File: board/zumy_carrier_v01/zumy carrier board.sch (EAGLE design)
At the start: 22 parts, among them IC1 SN74AUP2G17, IC2 SN74AUP2G17, J1 ODROID_POWER, J2 BATT_POWER, M2 ITG/MPU_MODULE, M3 POLOLU_DRV8833_MODULE, SW1 500SSP1S1M6QEA

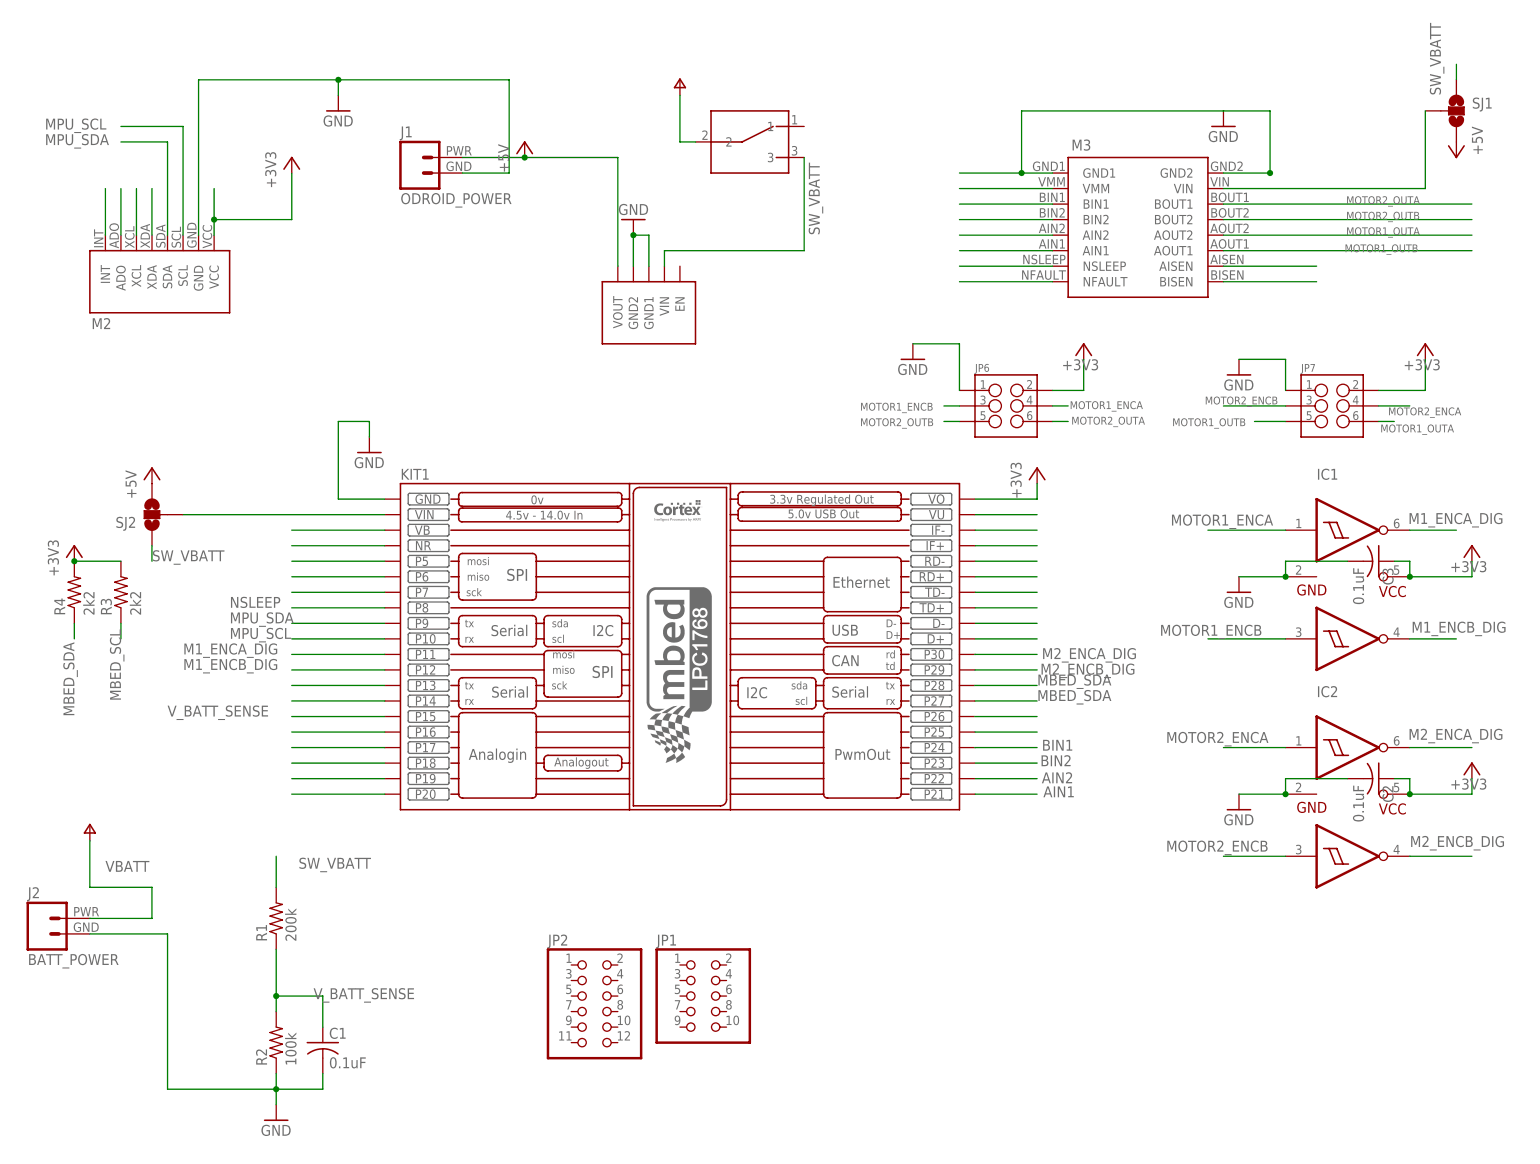
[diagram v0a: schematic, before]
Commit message: First pass at layout done
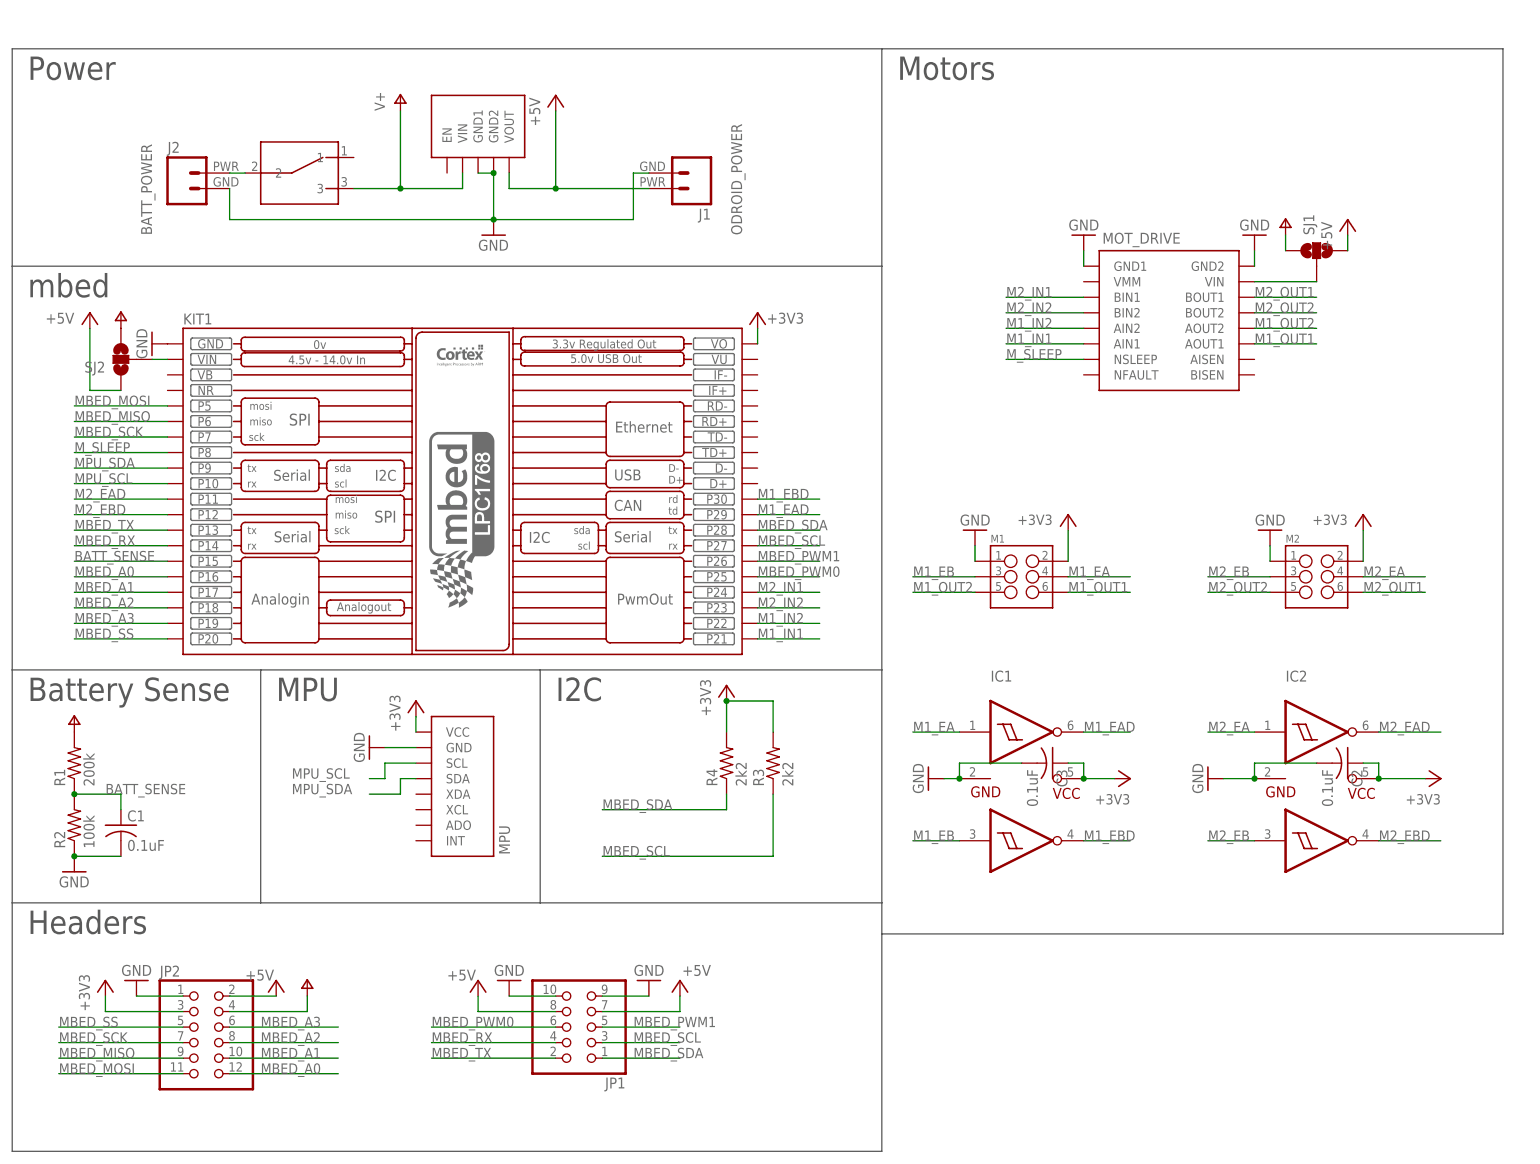
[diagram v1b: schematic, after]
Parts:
- removed JP6, JP7: (no value), SparkFun-Connectors:M03X2SHROUD
- removed M3: POLOLU_DRV8833_MODULE, zumy:POLOLU_DRV8833_MODULE
- added M1: (no value), SparkFun-Connectors:M03X2SHROUD
- added MOT_DRIVE: POLOLU_DRV8833_MODULE, zumy:POLOLU_DRV8833_MODULE
- added MPU: ITG/MPU_MODULE, zumy:ITG/MPU_MODULE
- M2: value ITG/MPU_MODULE -> (none); device zumy:ITG/MPU_MODULE -> SparkFun-Connectors:M03X2SHROUD
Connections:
- net VBATT renamed N$2
- net V_BATT_SENSE renamed BATT_SENSE
- removed net AIN1: KIT1.P21, M3.AIN1
- removed net AIN2: KIT1.P22, M3.AIN2
- removed net BIN1: KIT1.P24, M3.BIN1
- removed net BIN2: KIT1.P23, M3.BIN2
- removed net M1_ENCA_DIG: IC1.1Y, KIT1.P11
- removed net M1_ENCB_DIG: IC1.2Y, KIT1.P12
- removed net M2_ENCA_DIG: IC2.1Y, KIT1.P30
- removed net M2_ENCB_DIG: IC2.2Y, KIT1.P29
- removed net MOTOR1_ENCA: IC1.1A, JP6.4
- removed net MOTOR1_ENCB: IC1.2A, JP6.3
- removed net MOTOR1_OUTA: JP7.6, M3.AOUT2
- removed net MOTOR1_OUTB: JP7.5, M3.AOUT1
- removed net MOTOR2_ENCA: IC2.1A, JP7.4
- removed net MOTOR2_ENCB: IC2.2A, JP7.3
- removed net MOTOR2_OUTA: JP6.6, M3.BOUT1
- removed net MOTOR2_OUTB: JP6.5, M3.BOUT2
- removed net N$1 (its old number): M2.INT
- removed net N$10: KIT1.P16
- removed net N$11: KIT1.VB
- removed net N$12: KIT1.NR
- removed net N$13: KIT1.P5
- removed net N$14: KIT1.P6
- removed net N$15: KIT1.P7
- removed net N$16: M3.VIN, SJ1.2
- removed net N$2 (its old number): M2.ADO
- removed net N$21: KIT1.P13
- removed net N$22: KIT1.P14
- removed net N$25: KIT1.P17
- removed net N$26: KIT1.P18
- removed net N$27: KIT1.P19
- removed net N$33: KIT1.P25
- removed net N$34: KIT1.P26
- removed net N$4: M2.XDA
- removed net N$41: KIT1.TD+
- removed net N$42: KIT1.TD-
- removed net N$43: KIT1.RD+
- removed net N$44: KIT1.RD-
- removed net N$45: KIT1.IF+
- removed net N$46: KIT1.IF-
- removed net N$47: KIT1.VU
- removed net N$5: KIT1.D-
- removed net N$50: M3.VMM
- removed net N$56: M3.NFAULT
- removed net N$6: KIT1.D+
- removed net N$63: M3.AISEN
- removed net N$64: M3.BISEN
- removed net N$7: KIT1.P20
- removed net NSLEEP: KIT1.P8, M3.NSLEEP
- removed net SW_VBATT: R1.2, SJ1.1, SJ2.1, SW1.3, U$5.VIN
- new net M1_EA: IC1.1A, M1.4
- new net M1_EAD: IC1.1Y, KIT1.P29
- new net M1_EB: IC1.2A, M1.3
- new net M1_EBD: IC1.2Y, KIT1.P30
- new net M1_IN1: KIT1.P21, MOT_DRIVE.AIN1
- new net M1_IN2: KIT1.P22, MOT_DRIVE.AIN2
- new net M1_OUT1: M1.6, MOT_DRIVE.AOUT1
- new net M1_OUT2: M1.5, MOT_DRIVE.AOUT2
- new net M2_EA: IC2.1A, M2.4
- new net M2_EAD: IC2.1Y, KIT1.P11
- new net M2_EB: IC2.2A, M2.3
- new net M2_EBD: IC2.2Y, KIT1.P12
- new net M2_IN1: KIT1.P24, MOT_DRIVE.BIN1
- new net M2_IN2: KIT1.P23, MOT_DRIVE.BIN2
- new net M2_OUT1: M2.6, MOT_DRIVE.BOUT1
- new net M2_OUT2: M2.5, MOT_DRIVE.BOUT2
- new net MBED_A0: JP2.12, KIT1.P16
- new net MBED_A1: JP2.10, KIT1.P17
- new net MBED_A2: JP2.8, KIT1.P18
- new net MBED_A3: JP2.6, KIT1.P19
- new net MBED_MISO: JP2.9, KIT1.P6
- new net MBED_MOSI: JP2.11, KIT1.P5
- new net MBED_PWM0: JP1.6, KIT1.P25
- new net MBED_PWM1: JP1.5, KIT1.P26
- new net MBED_RX: JP1.4, KIT1.P14
- new net MBED_SCK: JP2.7, KIT1.P7
- new net MBED_SS: JP2.5, KIT1.P20
- new net MBED_TX: JP1.2, KIT1.P13
- new net M_SLEEP: KIT1.P8, MOT_DRIVE.NSLEEP
- new net V+: JP2.4, R1.2, SJ1.1, SJ2.3, SW1.3, U$5.VIN
- net +3V3: now also JP2.3, M1.2, M2.2, MPU.VCC; no longer JP6.2, JP7.2, M2.VCC
- net +5V: now also JP1.7, JP1.8, JP2.2, SJ2.1; no longer SJ2.3
- net GND: now also JP1.10, JP1.9, JP2.1, M1.1, M2.1, MOT_DRIVE.GND1, MOT_DRIVE.GND2, MPU.GND; no longer JP6.1, JP7.1, M2.GND, M3.GND1, M3.GND2
- net MBED_SCL: now also JP1.3
- net MBED_SDA: now also JP1.1
- net MPU_SCL: now also MPU.SCL; no longer M2.SCL
- net MPU_SDA: now also MPU.SDA; no longer M2.SDA
- net N$3: now also MOT_DRIVE.VIN, SJ1.2; no longer M2.XCL
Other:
- note added: "Battery Sense"
- note added: "Headers"
- note added: "I2C"
- note added: "MPU"
- note added: "Motors"
- note added: "Power"
- note added: "mbed"
- moved on the sheet: C1, C2, C3, IC1, IC2, J1, J2, JP1, JP2, KIT1, R1, R2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
